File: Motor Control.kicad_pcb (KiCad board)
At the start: 2 copper layers, 160 x 135.1 mm, 112 parts, among them J1 Conn_01x02_Socket, J4 Conn_01x02_Socket, J400 Conn_01x05_Pin, J410 Conn_01x06_Pin, J411 USB_B, J5 Conn_01x02_Socket, J6 Conn_01x02_Socket, Q110 IRLZ44N, Q111 BC557, Q112 BC547, Q113 BC557, Q120 IRLZ44N, Q121 BC557, Q122 BC547, Q123 BC557, Q130 IRLZ44N, Q131 BC547, Q132 BC557, Q140 IRLZ44N, Q141 BC547, Q142 BC557, Q210 BC547, Q220 BC547, Q230 BC547, Q240 BC547, SW310 RotaryEncoder_Switch_MP, U210 4N35, U220 4N35, U230 4N35, U240 4N35, U300 74AHC595, U400 PIC18F26K22-xSP, U410 MCP2221AxP, U900 LM317, U901 L78L05_TO92, U902 HCPL7510

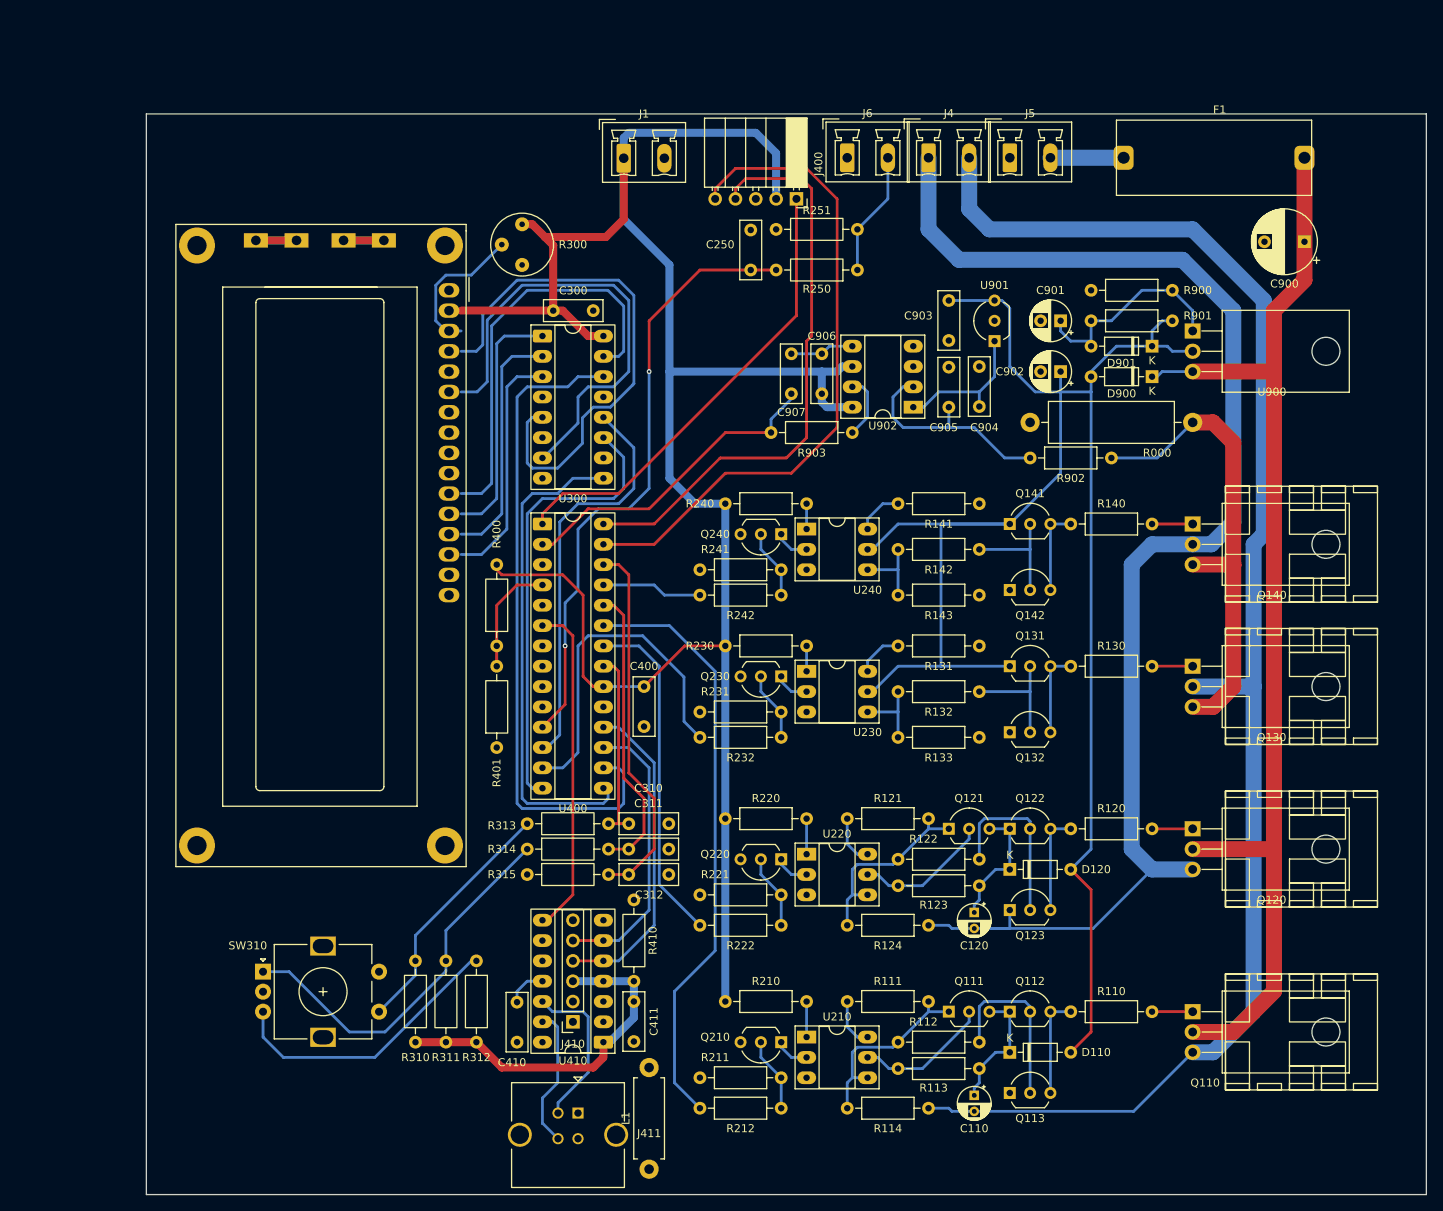
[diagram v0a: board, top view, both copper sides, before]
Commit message: V 1.0 fabrication output
V 1.0 ready for fabrication
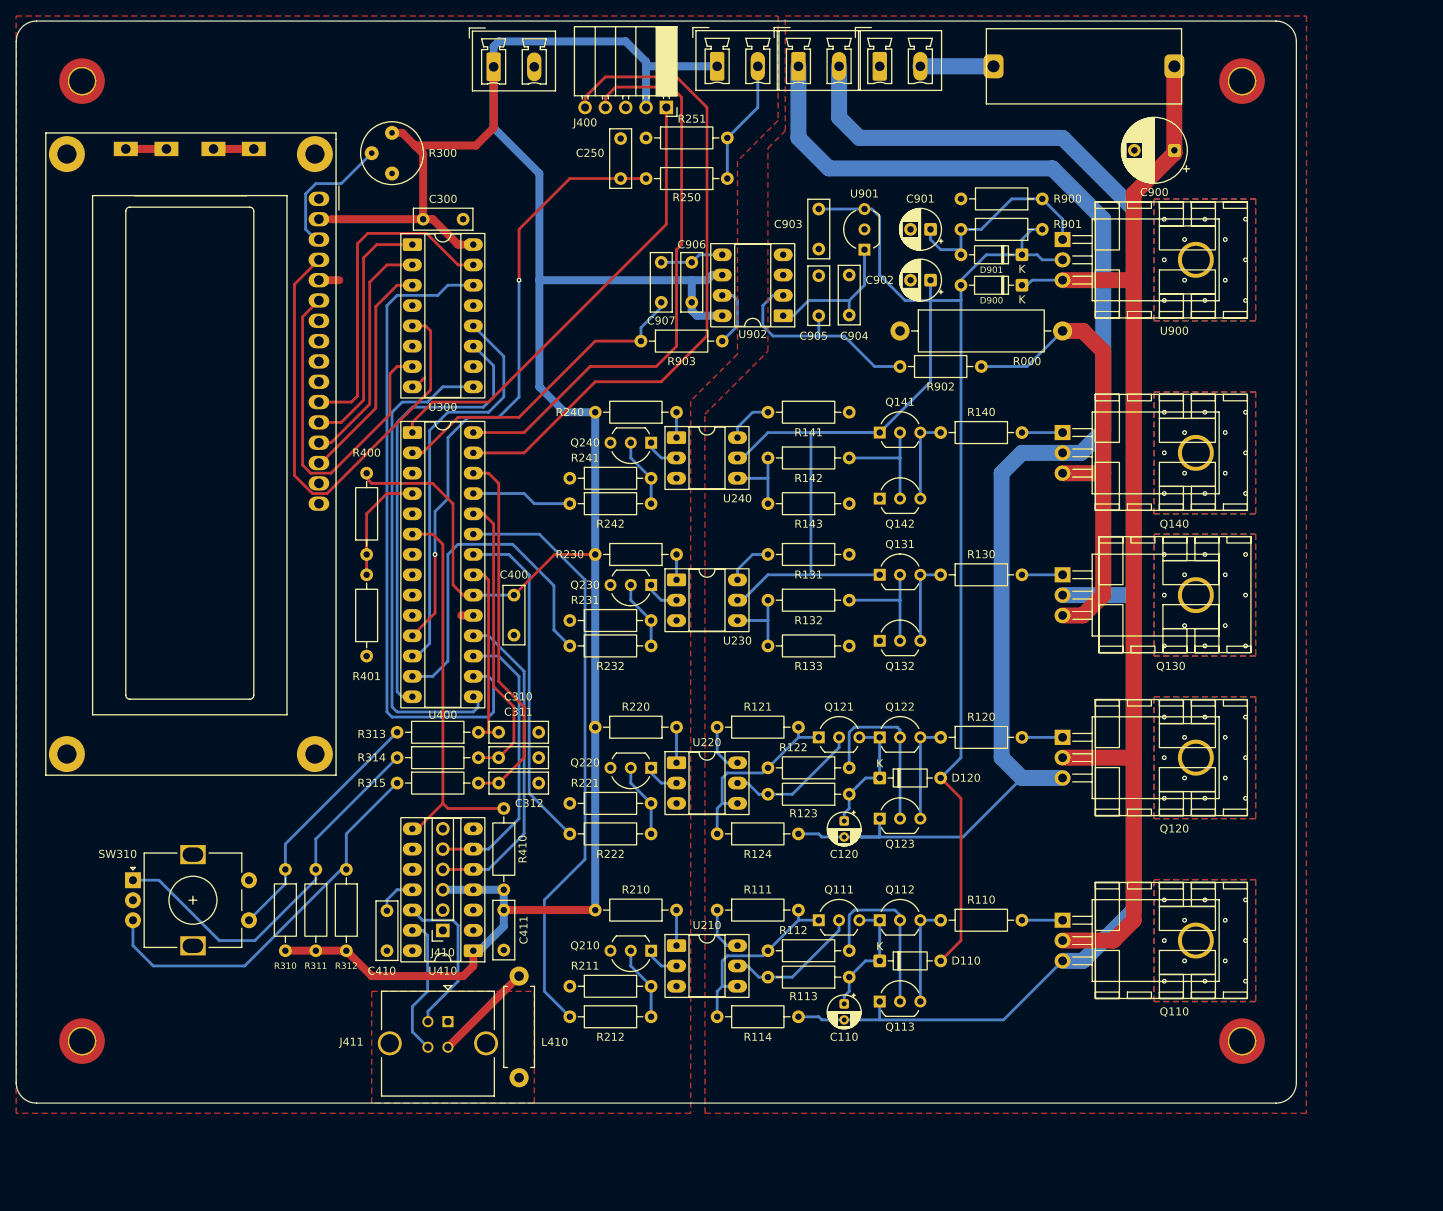
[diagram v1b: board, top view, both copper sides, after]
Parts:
- removed L1: L_Ferrite_Small, Resistor_THT:R_Axial_DIN0411_L9.9mm_D3.6mm_P12.70mm_Horizontal
- added G***: LOGO, User:logo, B.Cu at (84.1, 90.2)
- added L410: L_Ferrite_Small, Resistor_THT:R_Axial_DIN0411_L9.9mm_D3.6mm_P12.70mm_Horizontal, F.Cu at (126.6, 150.5)
- added REF**: Heatsink_Fisher_FK237SA220H, User:Heatsink_Fisher_FK237SA220O, F.Cu at (198.7, 55.5)
- added REF**: MountingHole_3.2mm_M3_ISO7380_Pad_TopOnly, MountingHole:MountingHole_3.2mm_M3_ISO7380_Pad_TopOnly, F.Cu at (72.0, 145.9)
- added REF**: MountingHole_3.2mm_M3_ISO7380_Pad_TopOnly, MountingHole:MountingHole_3.2mm_M3_ISO7380_Pad_TopOnly, F.Cu at (217.0, 145.9)
- added REF**: MountingHole_3.2mm_M3_ISO7380_Pad_TopOnly, MountingHole:MountingHole_3.2mm_M3_ISO7380_Pad_TopOnly, F.Cu at (72.0, 25.9)
- added REF**: MountingHole_3.2mm_M3_ISO7380_Pad_TopOnly, MountingHole:MountingHole_3.2mm_M3_ISO7380_Pad_TopOnly, F.Cu at (217.0, 25.9)
- Q110, Q120, Q130, Q140, U900: footprint Package_TO_SOT_THT:TO-220-3_Horizontal_TabDown -> User:TO-220-3_Horizontal_TabDown_HoleToCenter
- moved REF** 19.9 mm to (198.7, 79.6)
- moved D110 19.9 mm to (171.7, 135.9)
- moved Q112 19.9 mm to (171.7, 130.8)
- moved Q113 19.9 mm to (171.7, 141.0)
- moved Q131 19.9 mm to (171.7, 87.6)
- moved Q141 19.9 mm to (171.7, 69.8)
- moved R110 19.9 mm to (179.3, 130.8)
- moved R112 19.9 mm to (167.9, 134.6)
- moved R113 19.9 mm to (167.9, 137.9)
- moved R123 19.9 mm to (167.9, 115.1)
- moved R130 19.9 mm to (179.3, 87.6)
- moved R133 19.9 mm to (167.9, 96.5)
- moved R140 19.9 mm to (179.3, 69.8)
- moved R143 19.9 mm to (167.9, 78.7)
- moved C904 19.9 mm to (167.9, 55.2)
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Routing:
- net +5V: track 311.1 -> 331.4 mm
- net GNDD: track 8.01 -> 26.6 mm
- net Net-(DS300-E): track 57.8 -> 44.1 mm
- net Net-(R312-Pad1): track 35.9 -> 49.3 mm
- net Net-(DS300-D4): track 51.6 -> 40.8 mm
- net RA4: track 40.6 -> 48.5 mm
- net Net-(DS300-RS): track 66.8 -> 61.5 mm
- net /H Bridge/Out_{1}: track 191.0 -> 194.6 mm, vias 0 -> 12
- net Net-(DS300-VO): track 18.5 -> 16.6 mm
- net Net-(DS300-D7): track 29.9 -> 28.3 mm
- net +24V: track 143.7 -> 142.3 mm, vias 0 -> 24
- net Net-(DS300-D5): track 30.8 -> 31.3 mm
- net +12V: vias 0 -> 12
- net /H Bridge/Out_{2}: vias 0 -> 12
- added copper zone on B.Cu, net +12V
- added copper zone on F.Cu, net +12V
- added copper zone on B.Cu, net +24V
- added copper zone on F.Cu, net +24V
- added copper zone on B.Cu, net /H Bridge/Out_{1}
- added copper zone on F.Cu, net /H Bridge/Out_{1}
- added copper zone on B.Cu, net /H Bridge/Out_{2}
- added copper zone on F.Cu, net /H Bridge/Out_{2}
- added copper zone on F.Cu, net GNDD
- added copper zone on F.Cu, net GNDPWR
- added copper zone on F.Cu, net Net-(J411-Shield)
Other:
- board size 160 x 135.1 mm -> 160 x 135.3 mm
- board text added: "Motor Control v 1.0"
